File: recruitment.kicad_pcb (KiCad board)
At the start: 2 copper layers, 18 parts, among them Q1 BSN20, SW1 SW_SPST

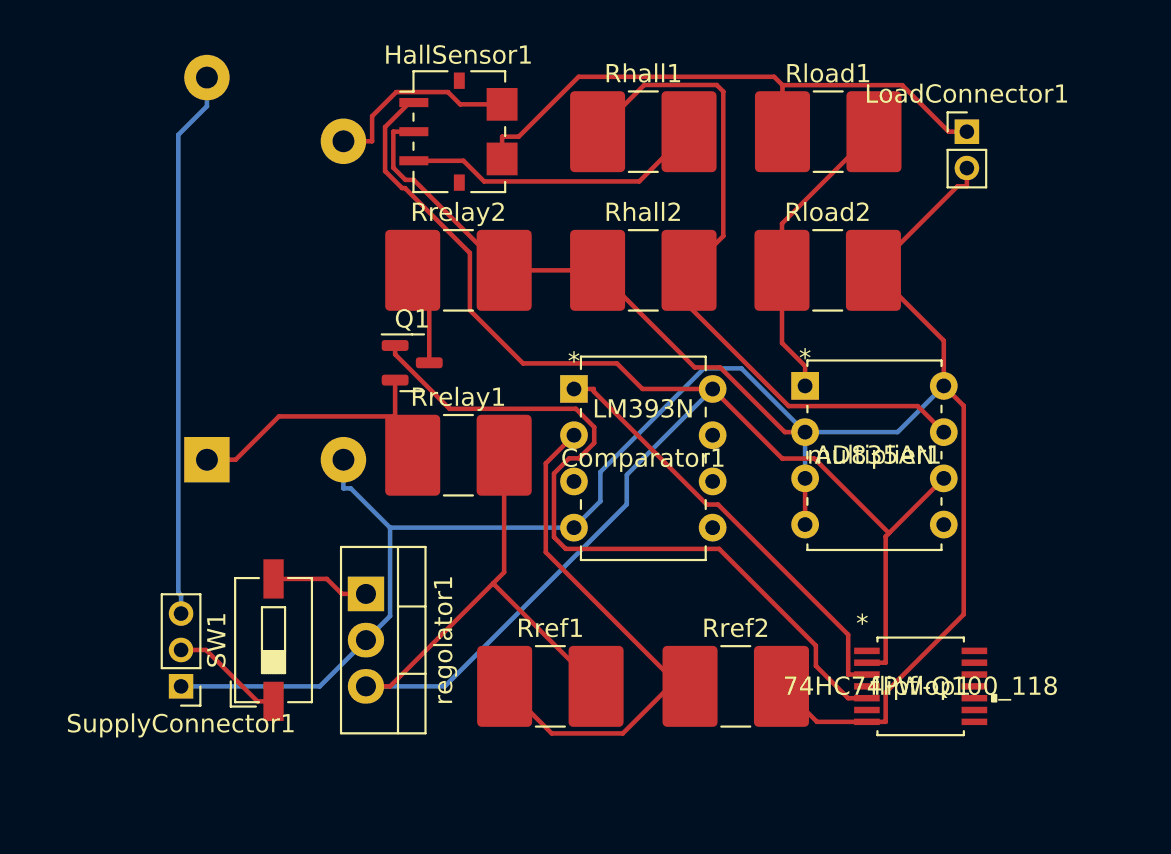
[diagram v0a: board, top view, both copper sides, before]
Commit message: check
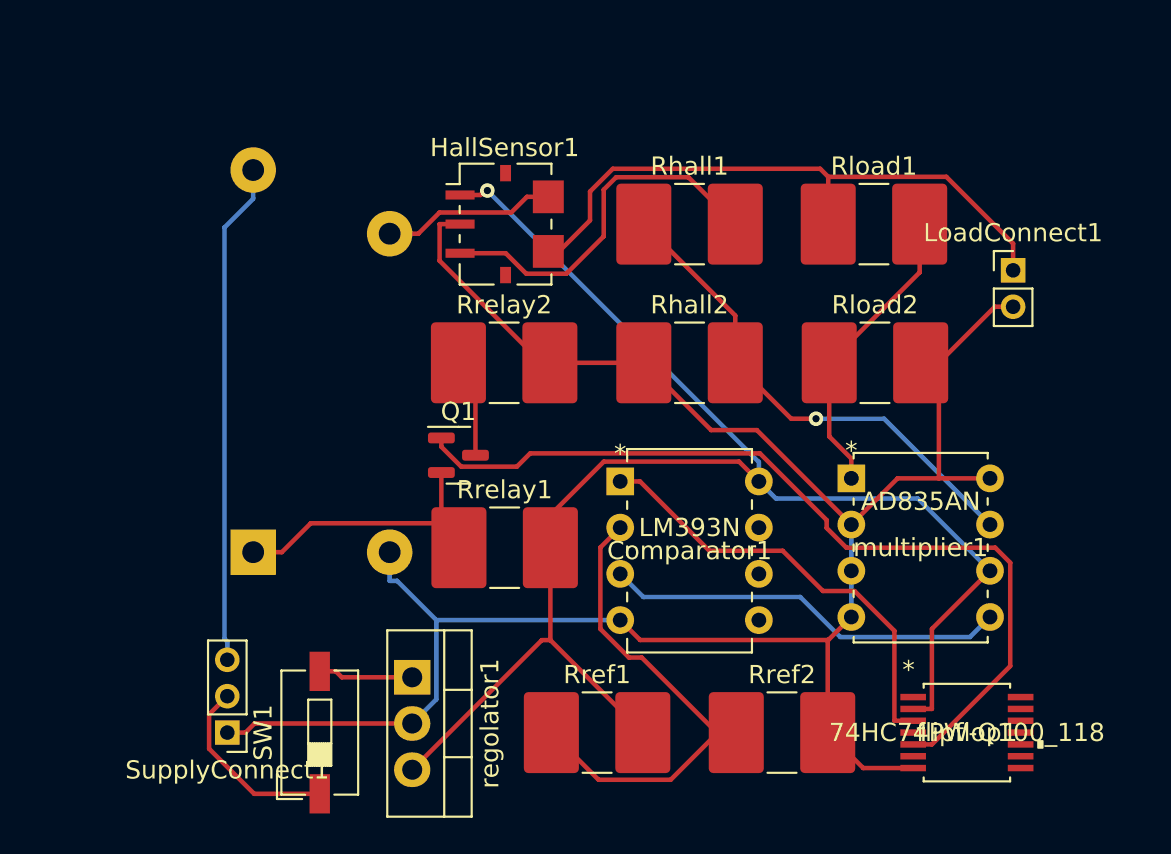
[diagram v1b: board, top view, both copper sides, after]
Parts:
- removed LoadConnector1: Conn_01x02_Female, Connector_PinHeader_2.00mm:PinHeader_1x02_P2.00mm_Vertical
- removed SupplyConnector1: Conn_01x03_Female, Connector_PinHeader_2.00mm:PinHeader_1x03_P2.00mm_Vertical
- added LoadConnect1: Conn_01x02_Female, Connector_PinHeader_2.00mm:PinHeader_1x02_P2.00mm_Vertical, F.Cu at (154.9, 83.8)
- added SupplyConnect1: Conn_01x03_Female, Connector_PinHeader_2.00mm:PinHeader_1x03_P2.00mm_Vertical, F.Cu at (111.8, 109.2)
- Rrelay1: value R -> 10
- Rrelay2: value R -> 15
- SW1: value SW_SPST -> switch
- moved Rload2 5.70 mm to (147.3, 88.9)
- moved Rhall2 5.68 mm to (137.2, 88.9)
- moved multiplier1 5.68 mm to (146.1, 95.2)
- moved HallSensor1 5.68 mm to (127.0, 81.3)
- moved Relay1 5.68 mm to (113.2, 99.3)
- moved Rrelay1 5.68 mm to (127.0, 99.1)
- moved SW1 5.68 mm to (116.8, 109.2)
- moved Comparator1 5.68 mm to (133.3, 95.4)
- moved Q1 5.68 mm to (124.5, 94.0)
- moved Rhall1 5.68 mm to (137.2, 81.3)
- moved Rrelay2 5.67 mm to (127.0, 88.9)
- moved Rload1 5.67 mm to (147.3, 81.3)
- moved regolator1 5.24 mm to (121.9, 106.2)
- moved Rref1 3.61 mm to (132.1, 109.2)
- moved Rref2 3.59 mm to (142.2, 109.2)
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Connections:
- Comparator1 pad 3: unconnected-(Comparator1-Pad3) -> /V_pot
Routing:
- net GND: track 140.5 -> 114.2 mm
- net /V_pot: track 0.00 -> 22.2 mm
- net /Vcc: track 106.2 -> 86.2 mm, vias 0 -> 1
- net /V_Nhall: track 37.6 -> 27.4 mm, vias 0 -> 1
- net /V_ff: track 41.9 -> 48.0 mm
- net Net-(SW1-Pad1): track 6.25 -> 10.4 mm
- net Net-(HallSensor1-Pad3): track 16.7 -> 20.4 mm
- net Net-(Relay1-Pad3): track 30.2 -> 27.6 mm
- net /V_ref: track 29.6 -> 27.1 mm
- net Net-(HallSensor1-Pad5): track 31.9 -> 34.1 mm
- net Net-(HallSensor1-Pad6): track 10.9 -> 9.56 mm
